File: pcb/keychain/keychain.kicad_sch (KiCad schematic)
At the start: 11 parts, among them J2 AVR-ISP-6, J3 Vin, U1 ATtiny84A-SS, U3 LM1117MP-3.3

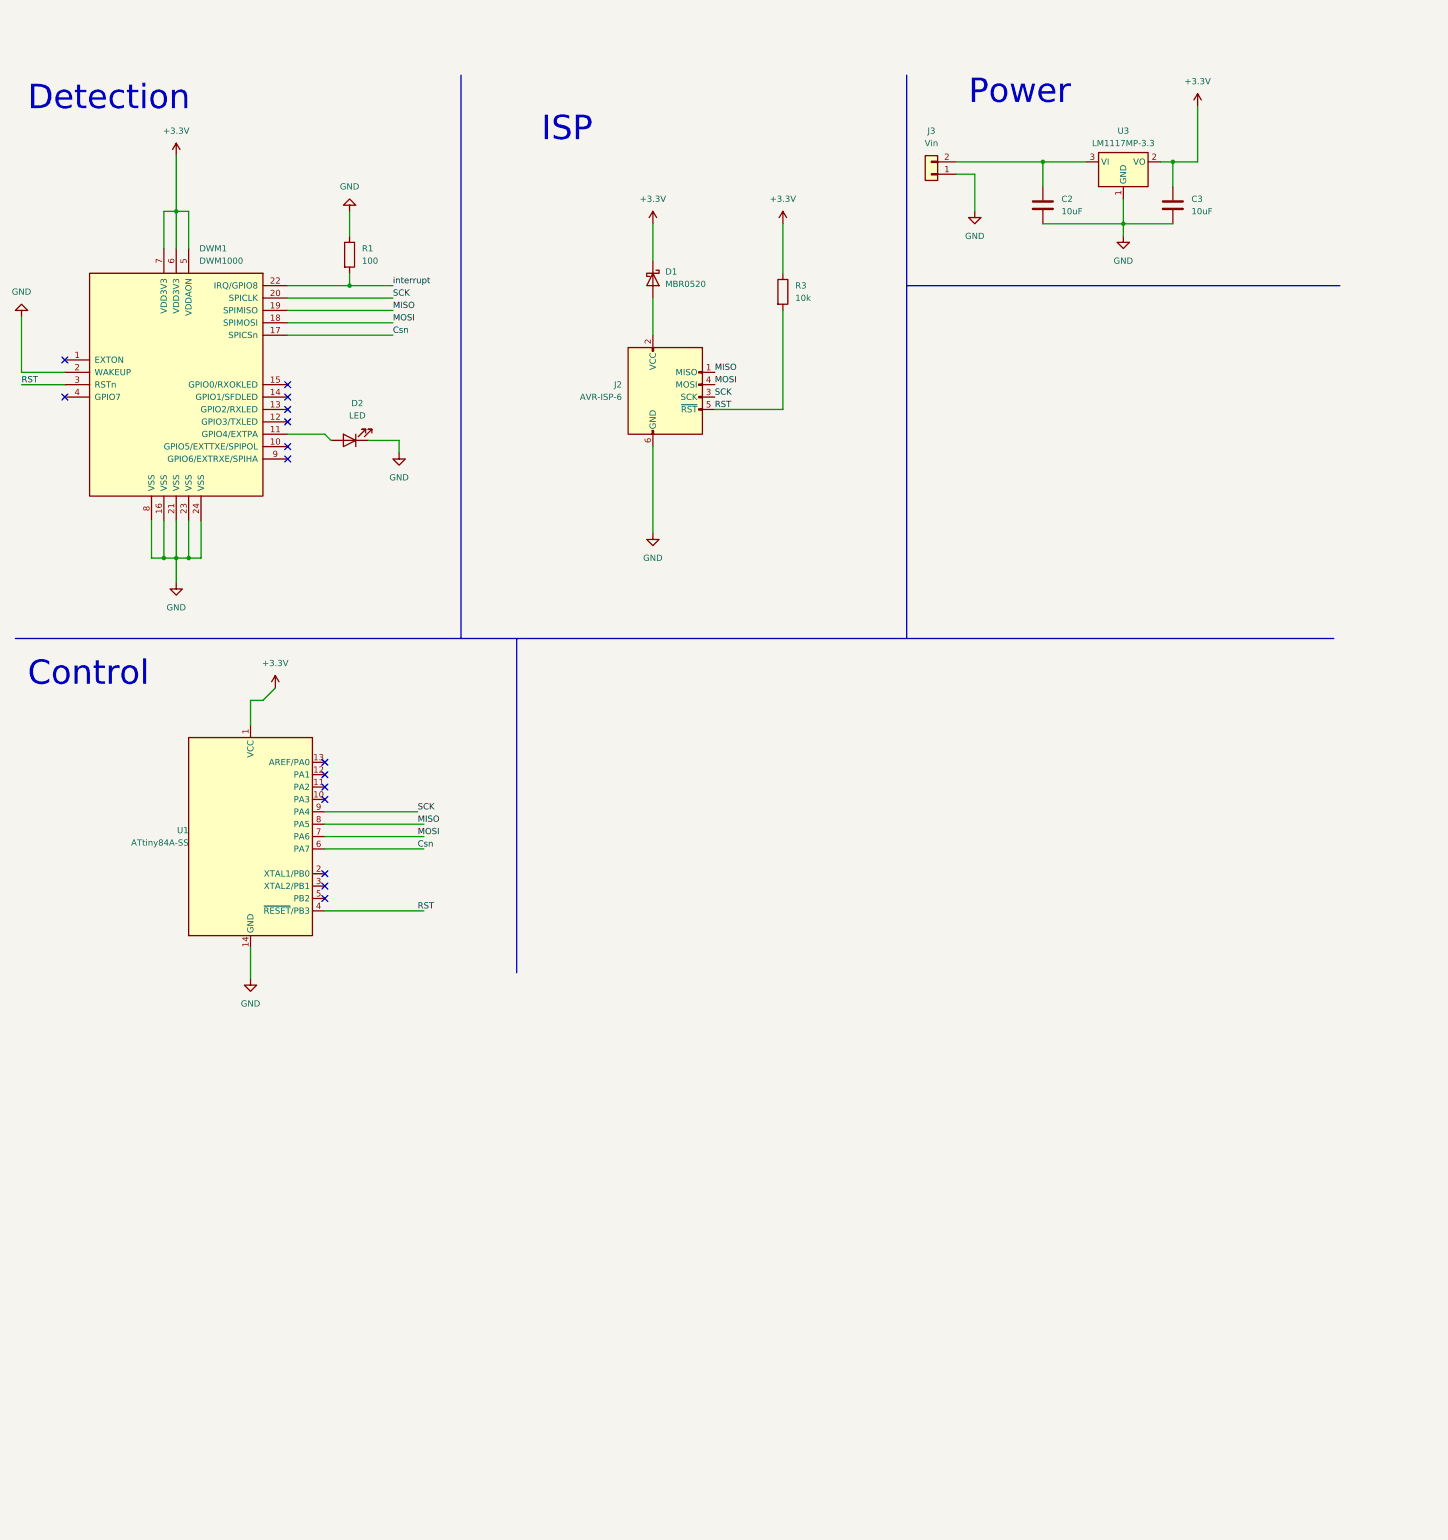
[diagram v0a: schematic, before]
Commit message: dish pcb updated
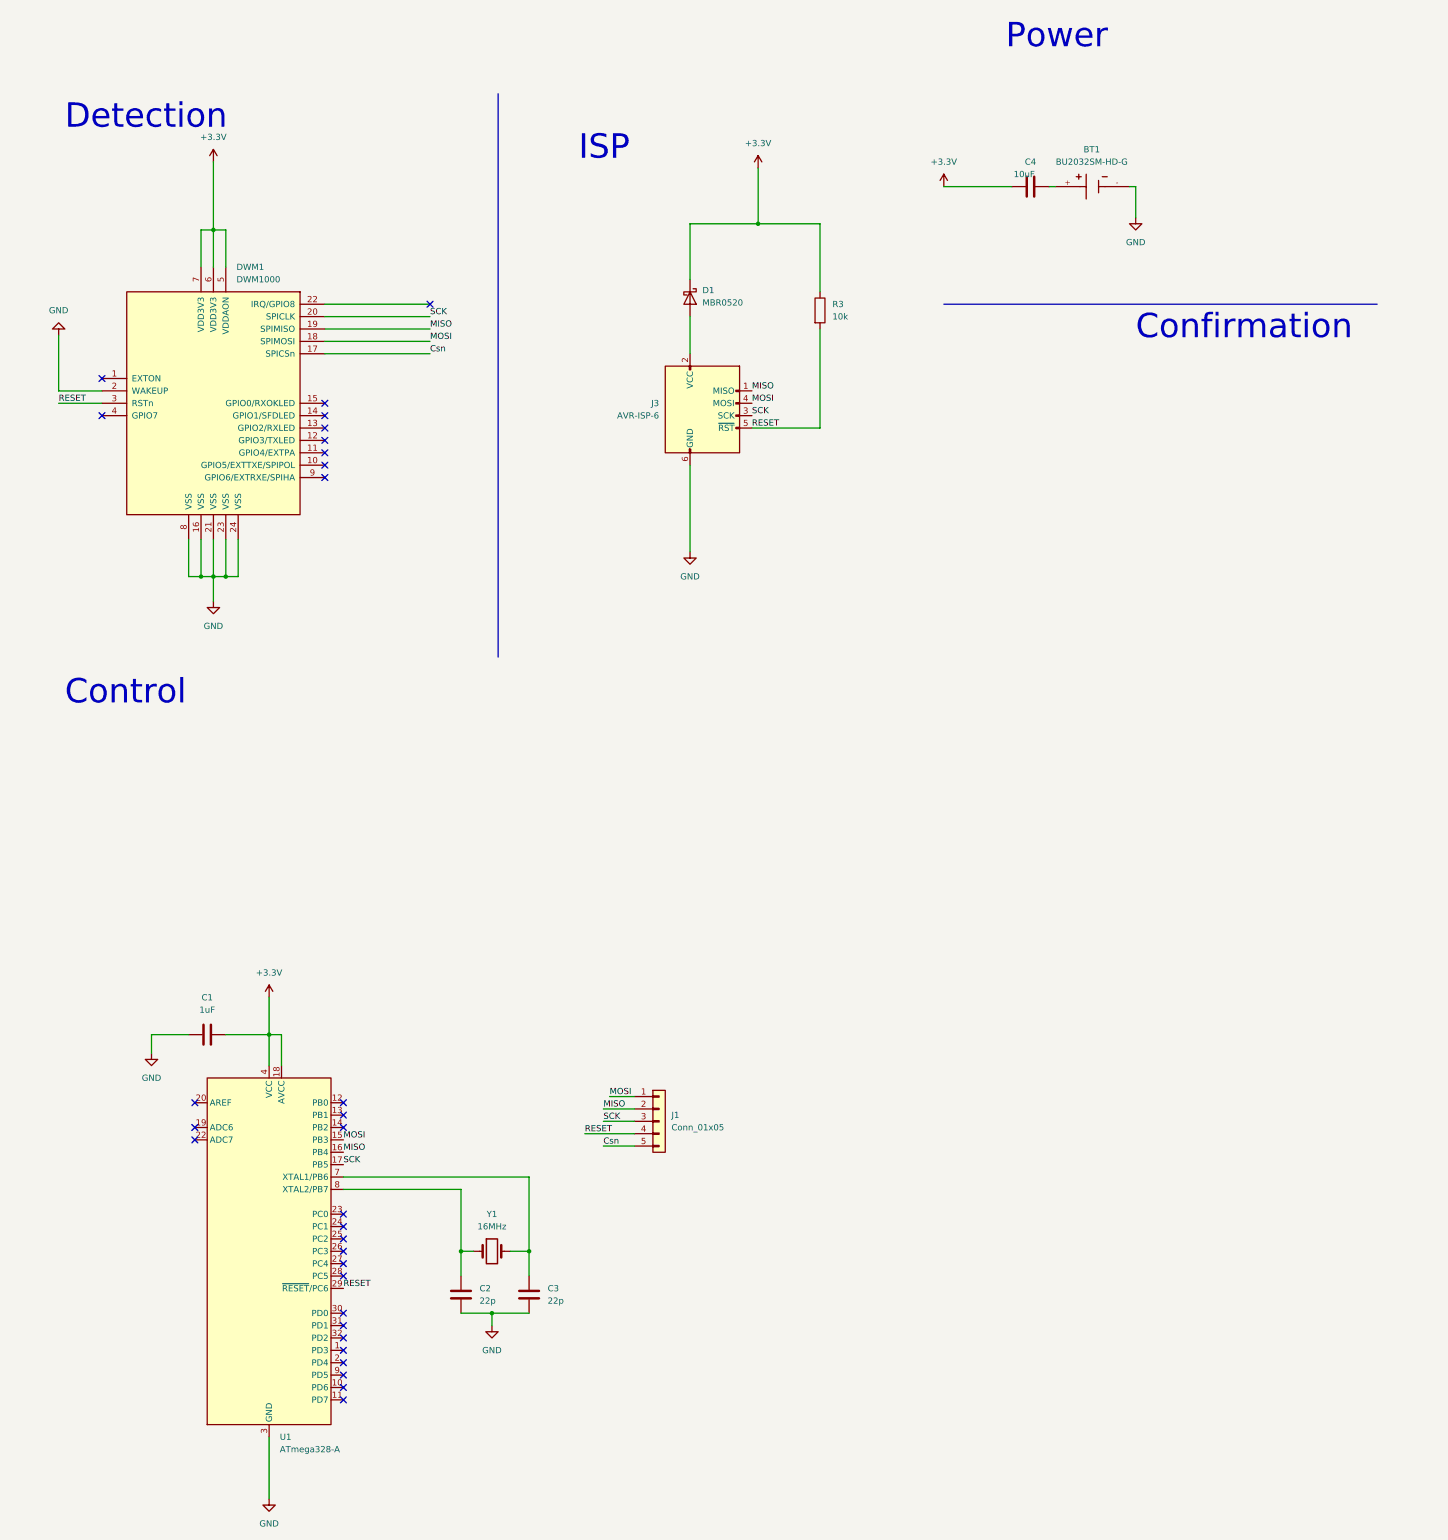
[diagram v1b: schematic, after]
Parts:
- removed D2: LED, LED_SMD:LED_0805_2012Metric_Pad1.15x1.40mm_HandSolder, symbol Device:LED
- removed J2: AVR-ISP-6, Connector_IDC:IDC-Header_2x03_P2.54mm_Vertical, symbol Connector:AVR-ISP-6
- removed J3: Vin, Connector_Molex:Molex_KK-254_AE-6410-02A_1x02_P2.54mm_Vertical, symbol Connector_Generic:Conn_01x02
- removed R1: 100, Resistor_SMD:R_0805_2012Metric_Pad1.20x1.40mm_HandSolder, symbol Device:R
- removed U1: ATtiny84A-SS, Package_SO:SOIC-14_3.9x8.7mm_P1.27mm, symbol MCU_Microchip_ATtiny:ATtiny84A-SS
- removed U3: LM1117MP-3.3, Package_TO_SOT_SMD:SOT-223-3_TabPin2, symbol Regulator_Linear:LM1117MP-3.3
- added BT1: BU2032SM-HD-G, BU2032SM-HD-G:BAT_BU2032SM-HD-G, symbol BU2032SM-HD-G:BU2032SM-HD-G
- added C1: 1uF, Capacitor_SMD:C_0805_2012Metric_Pad1.18x1.45mm_HandSolder, symbol Device:C
- added C4: 10uF, Capacitor_SMD:C_0805_2012Metric_Pad1.18x1.45mm_HandSolder, symbol Device:C
- added J1: Conn_01x05, Connector_Molex:Molex_KK-254_AE-6410-05A_1x05_P2.54mm_Vertical, symbol Connector_Generic:Conn_01x05
- added J3: AVR-ISP-6, Connector_IDC:IDC-Header_2x03_P2.54mm_Vertical, symbol Connector:AVR-ISP-6
- added U1: ATmega328-A, Package_QFP:TQFP-32_7x7mm_P0.8mm, symbol MCU_Microchip_ATmega:ATmega328-A
- added Y1: 16MHz, Crystal:Crystal_HC49-U_Vertical, symbol Device:Crystal
- C2, C3: value 10uF -> 22p
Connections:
- net +3.3V: now also C1.2, C4.1, U1.18 (AVCC), U1.4 (VCC), U1.6 (VCC); no longer C3.1
- net Csn: now also J1.5 (Pin_5)
- net GND: now also BT1.-, C1.1, J3.6 (GND), U1.21 (GND), U1.3 (GND), U1.5 (GND)
- net MISO: now also J1.2 (Pin_2), J3.1 (MISO), U1.16 (PB4)
- net MOSI: now also J1.1 (Pin_1), J3.4 (MOSI), U1.15 (PB3)
- net SCK: now also J1.3 (Pin_3), J3.3 (SCK), U1.17 (PB5)
- net at C2.1: now also U1.8 (XTAL2/PB7), Y1.1
- net at D1.2 (A): now also J3.2 (VCC)
- net RST renamed RESET
- net RESET: now also J1.4 (Pin_4), J3.5 (~{RST}), U1.29 (~{RESET}/PC6)
- net interrupt: no longer names the net of DWM1.22 (IRQ/GPIO8)
- new net: BT1.+, C4.2
- new net: C3.1, U1.7 (XTAL1/PB6), Y1.2
- no-connect marks 15 -> 30
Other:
- note added: "Confirmation"
